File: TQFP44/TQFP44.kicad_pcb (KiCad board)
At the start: 2 copper layers, 56.1 x 20.6 mm, 12 parts, among them J1 Conn_01x22, J2 Conn_01x22, J3 Conn_02x22_Counter_Clockwise, J4 Conn_02x22_Counter_Clockwise_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, J5 Conn_02x22_Counter_Clockwise, J6 Conn_01x06

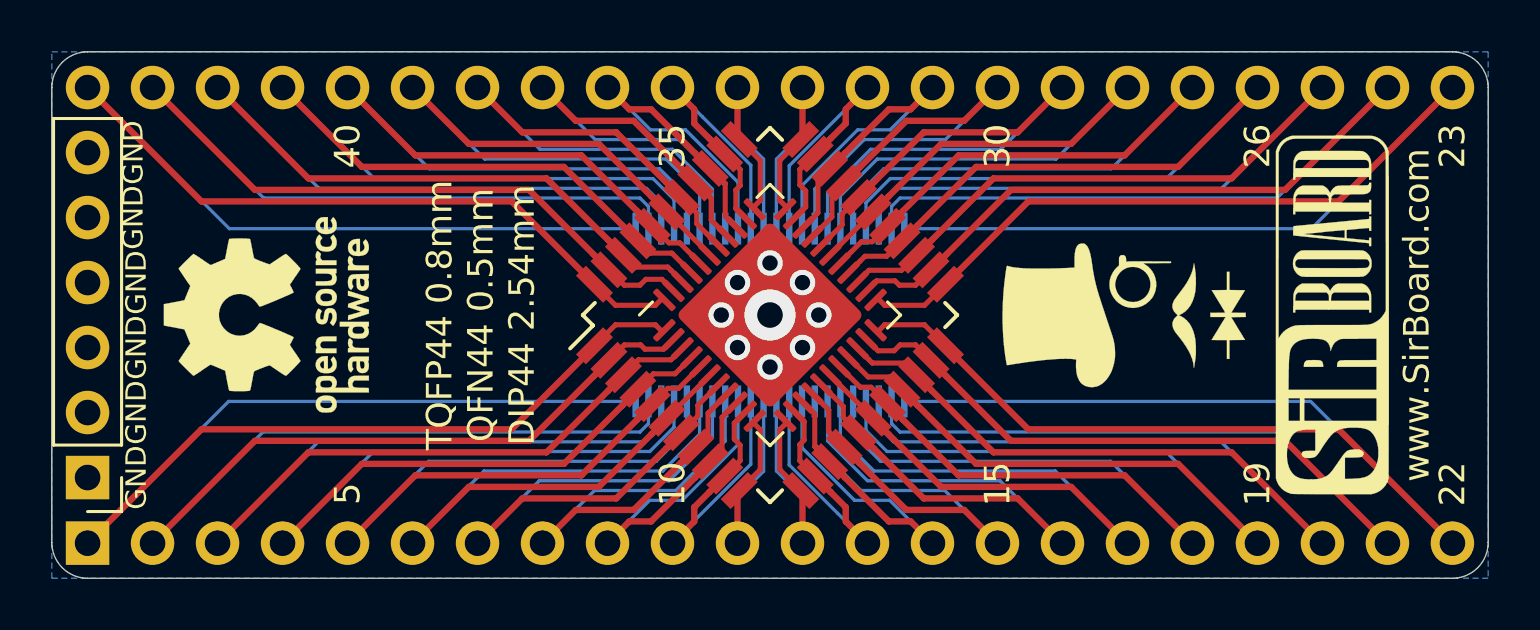
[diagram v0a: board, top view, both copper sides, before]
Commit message: Final Revisions
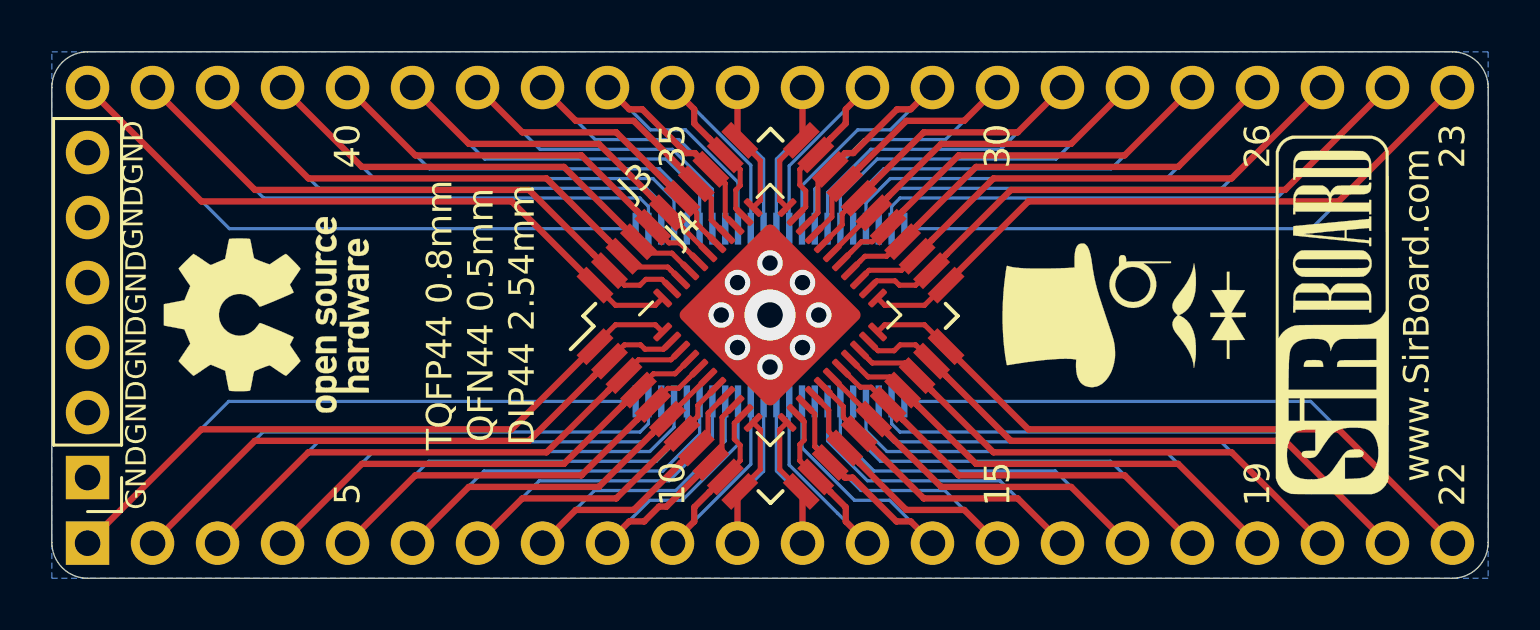
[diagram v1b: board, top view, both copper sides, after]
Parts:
- J4: value Conn_02x22_Counter_Clockwise_MountingPin -> Conn_02x22_Counter_Clockwise; footprint Package_DFN_QFN:QFN-44-1EP_7x7mm_P0.5mm_EP5.2x5.2mm -> Package_DFN_QFN:QFN-44-1EP_7x7mm_P0.5mm_EP5.15x5.15mm
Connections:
- J4 pad 45: Net-(J4-PadMP) -> (no net)
- J6 pad 1: Net-(J4-PadMP) -> Net-(J6-Pad1)
- J6 pad 2: Net-(J4-PadMP) -> Net-(J6-Pad1)
- J6 pad 3: Net-(J4-PadMP) -> Net-(J6-Pad1)
- J6 pad 4: Net-(J4-PadMP) -> Net-(J6-Pad1)
- J6 pad 5: Net-(J4-PadMP) -> Net-(J6-Pad1)
- J6 pad 6: Net-(J4-PadMP) -> Net-(J6-Pad1)
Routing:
- net Net-(J2-Pad9): track 2.64 -> 16.4 mm
- net Net-(J1-Pad14): track 30.0 -> 16.3 mm
- net Net-(J2-Pad10): track 2.95 -> 13.2 mm
- net Net-(J1-Pad13): track 23.4 -> 13.2 mm
- net Net-(J1-Pad9): track 7.96 -> 16.4 mm
- net Net-(J2-Pad14): track 24.9 -> 16.4 mm
- net Net-(J2-Pad13): track 20.0 -> 13.1 mm
- net Net-(J1-Pad10): track 6.34 -> 13.1 mm
- net Net-(J4-PadMP): vias 9 -> 0
- net (no net): vias 0 -> 9
- added copper zone on B.Cu, net Net-(J6-Pad1)
- removed copper zone on B.Cu, net Net-(J4-PadMP)
